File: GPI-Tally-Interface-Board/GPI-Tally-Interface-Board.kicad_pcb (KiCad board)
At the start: 2 copper layers, 155 x 90 mm, 44 parts, among them J1 DB25_Female, J2 DB25_Female, J20 AMP171826-4, J8 THD-20-R, SW1 SW_Push_45deg, SW10 SW_Push_45deg, SW11 SW_Push_45deg, SW12 SW_Push_45deg, SW13 SW_Push_45deg, SW14 SW_Push_45deg, SW15 SW_Push_45deg, SW16 SW_Push_45deg, SW2 SW_Push_45deg, SW3 SW_Push_45deg, SW4 SW_Push_45deg, SW5 SW_Push_45deg, SW6 SW_Push_45deg, SW7 SW_Push_45deg, SW8 SW_Push_45deg, SW9 SW_Push_45deg, U1 BOB-12009, U2 BOB-12009, U3 BOB-12009, U4 BOB-12009

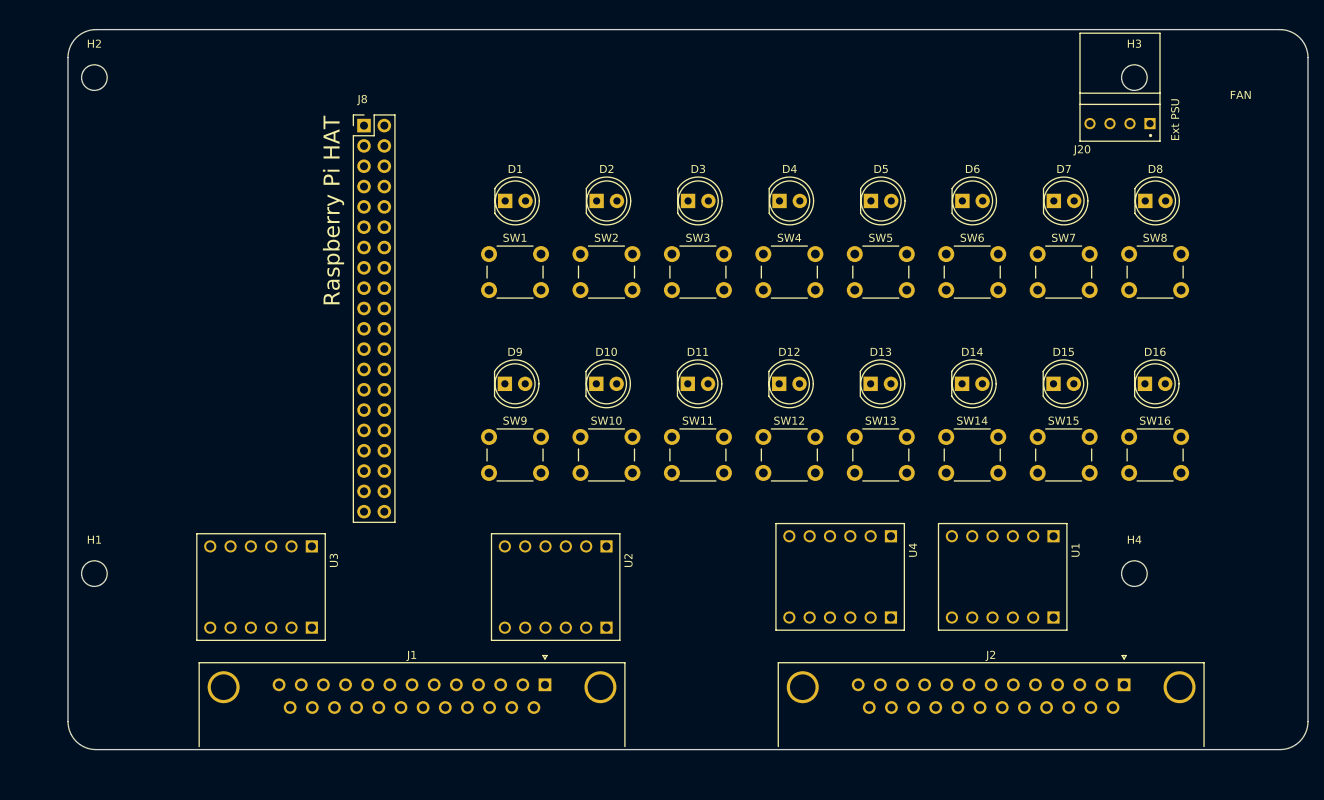
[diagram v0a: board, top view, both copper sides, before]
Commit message: oppto added
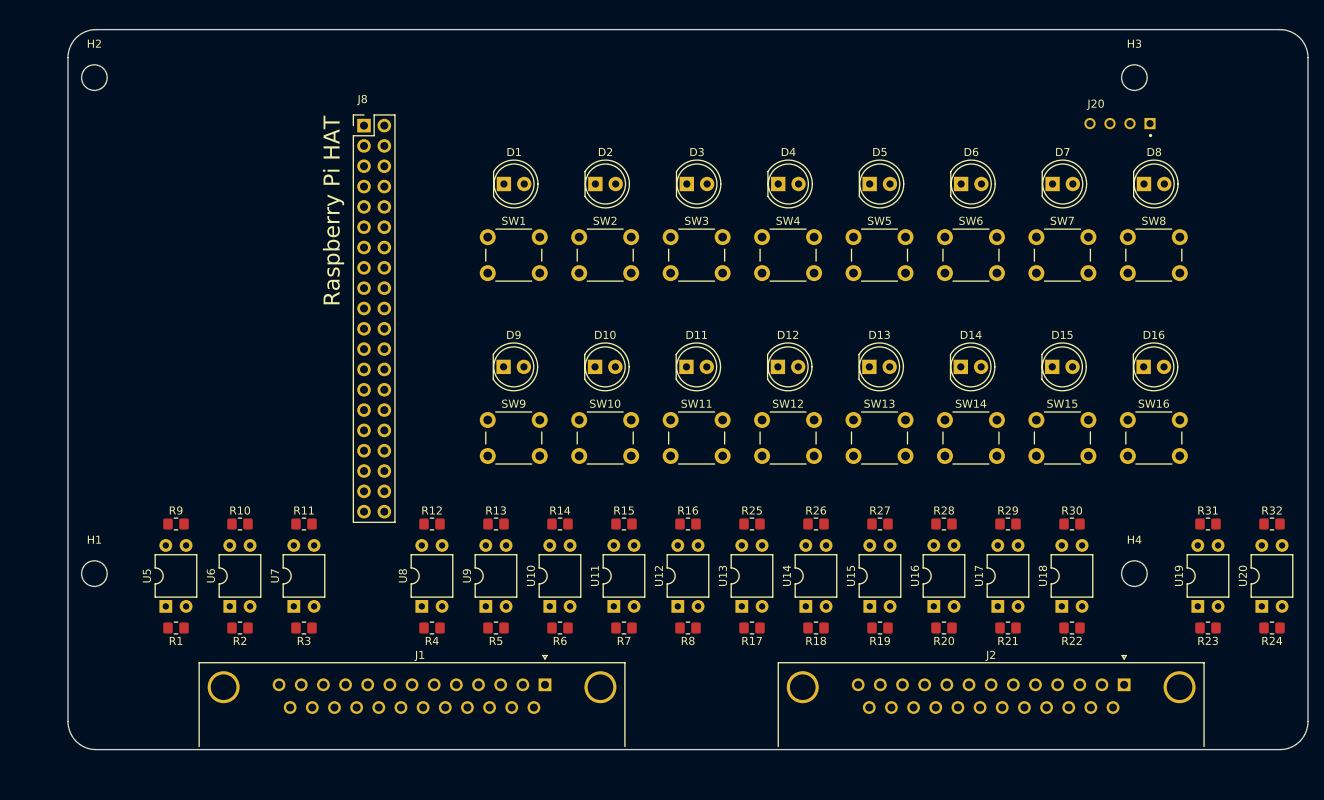
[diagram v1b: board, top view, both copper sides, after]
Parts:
- removed U1, U2, U3, U4: BOB-12009, BOB-12009:CONV_BOB-12009
- added R1: 470, Resistor_SMD:R_0805_2012Metric_Pad1.20x1.40mm_HandSolder, F.Cu at (77.0, 124.5)
- added R10: 470, Resistor_SMD:R_0805_2012Metric_Pad1.20x1.40mm_HandSolder, F.Cu at (85.0, 111.5)
- added R11: 470, Resistor_SMD:R_0805_2012Metric_Pad1.20x1.40mm_HandSolder, F.Cu at (93.0, 111.5)
- added R12: 470, Resistor_SMD:R_0805_2012Metric_Pad1.20x1.40mm_HandSolder, F.Cu at (109.0, 111.5)
- added R13: 470, Resistor_SMD:R_0805_2012Metric_Pad1.20x1.40mm_HandSolder, F.Cu at (117.0, 111.5)
- added R14: 470, Resistor_SMD:R_0805_2012Metric_Pad1.20x1.40mm_HandSolder, F.Cu at (125.0, 111.5)
- added R15: 470, Resistor_SMD:R_0805_2012Metric_Pad1.20x1.40mm_HandSolder, F.Cu at (133.0, 111.5)
- added R16: 470, Resistor_SMD:R_0805_2012Metric_Pad1.20x1.40mm_HandSolder, F.Cu at (141.0, 111.5)
- added R17: 470, Resistor_SMD:R_0805_2012Metric_Pad1.20x1.40mm_HandSolder, F.Cu at (149.0, 124.5)
- added R18: 470, Resistor_SMD:R_0805_2012Metric_Pad1.20x1.40mm_HandSolder, F.Cu at (157.0, 124.5)
- added R19: 470, Resistor_SMD:R_0805_2012Metric_Pad1.20x1.40mm_HandSolder, F.Cu at (165.0, 124.5)
- added R2: 470, Resistor_SMD:R_0805_2012Metric_Pad1.20x1.40mm_HandSolder, F.Cu at (85.0, 124.5)
- added R20: 470, Resistor_SMD:R_0805_2012Metric_Pad1.20x1.40mm_HandSolder, F.Cu at (173.0, 124.5)
- added R21: 470, Resistor_SMD:R_0805_2012Metric_Pad1.20x1.40mm_HandSolder, F.Cu at (181.0, 124.5)
- added R22: 470, Resistor_SMD:R_0805_2012Metric_Pad1.20x1.40mm_HandSolder, F.Cu at (189.0, 124.5)
- added R23: 470, Resistor_SMD:R_0805_2012Metric_Pad1.20x1.40mm_HandSolder, F.Cu at (206.0, 124.5)
- added R24: 470, Resistor_SMD:R_0805_2012Metric_Pad1.20x1.40mm_HandSolder, F.Cu at (214.0, 124.5)
- added R25: 470, Resistor_SMD:R_0805_2012Metric_Pad1.20x1.40mm_HandSolder, F.Cu at (149.0, 111.5)
- added R26: 470, Resistor_SMD:R_0805_2012Metric_Pad1.20x1.40mm_HandSolder, F.Cu at (157.0, 111.5)
- added R27: 470, Resistor_SMD:R_0805_2012Metric_Pad1.20x1.40mm_HandSolder, F.Cu at (165.0, 111.5)
- added R28: 470, Resistor_SMD:R_0805_2012Metric_Pad1.20x1.40mm_HandSolder, F.Cu at (173.0, 111.5)
- added R29: 470, Resistor_SMD:R_0805_2012Metric_Pad1.20x1.40mm_HandSolder, F.Cu at (181.0, 111.5)
- added R3: 470, Resistor_SMD:R_0805_2012Metric_Pad1.20x1.40mm_HandSolder, F.Cu at (93.0, 124.5)
- added R30: 470, Resistor_SMD:R_0805_2012Metric_Pad1.20x1.40mm_HandSolder, F.Cu at (189.0, 111.5)
- added R31: 470, Resistor_SMD:R_0805_2012Metric_Pad1.20x1.40mm_HandSolder, F.Cu at (206.0, 111.5)
- added R32: 470, Resistor_SMD:R_0805_2012Metric_Pad1.20x1.40mm_HandSolder, F.Cu at (214.0, 111.5)
- added R4: 470, Resistor_SMD:R_0805_2012Metric_Pad1.20x1.40mm_HandSolder, F.Cu at (109.0, 124.5)
- added R5: 470, Resistor_SMD:R_0805_2012Metric_Pad1.20x1.40mm_HandSolder, F.Cu at (117.0, 124.5)
- added R6: 470, Resistor_SMD:R_0805_2012Metric_Pad1.20x1.40mm_HandSolder, F.Cu at (125.0, 124.5)
- added R7: 470, Resistor_SMD:R_0805_2012Metric_Pad1.20x1.40mm_HandSolder, F.Cu at (133.0, 124.5)
- added R8: 470, Resistor_SMD:R_0805_2012Metric_Pad1.20x1.40mm_HandSolder, F.Cu at (141.0, 124.5)
- added R9: 470, Resistor_SMD:R_0805_2012Metric_Pad1.20x1.40mm_HandSolder, F.Cu at (77.0, 111.5)
- added U10: EL817, Package_DIP:DIP-4_W7.62mm, F.Cu at (123.7, 121.8)
- added U11: EL817, Package_DIP:DIP-4_W7.62mm, F.Cu at (131.7, 121.8)
- added U12: EL817, Package_DIP:DIP-4_W7.62mm, F.Cu at (139.7, 121.8)
- added U13: EL817, Package_DIP:DIP-4_W7.62mm, F.Cu at (147.7, 121.8)
- added U14: EL817, Package_DIP:DIP-4_W7.62mm, F.Cu at (155.7, 121.8)
- added U15: EL817, Package_DIP:DIP-4_W7.62mm, F.Cu at (163.7, 121.8)
- added U16: EL817, Package_DIP:DIP-4_W7.62mm, F.Cu at (171.7, 121.8)
- added U17: EL817, Package_DIP:DIP-4_W7.62mm, F.Cu at (179.7, 121.8)
- added U18: EL817, Package_DIP:DIP-4_W7.62mm, F.Cu at (187.7, 121.8)
- added U19: EL817, Package_DIP:DIP-4_W7.62mm, F.Cu at (204.7, 121.8)
- added U20: EL817, Package_DIP:DIP-4_W7.62mm, F.Cu at (212.7, 121.8)
- added U5: EL817, Package_DIP:DIP-4_W7.62mm, F.Cu at (75.7, 121.8)
- added U6: EL817, Package_DIP:DIP-4_W7.62mm, F.Cu at (83.7, 121.8)
- added U7: EL817, Package_DIP:DIP-4_W7.62mm, F.Cu at (91.7, 121.8)
- added U8: EL817, Package_DIP:DIP-4_W7.62mm, F.Cu at (107.7, 121.8)
- added U9: EL817, Package_DIP:DIP-4_W7.62mm, F.Cu at (115.7, 121.8)
- moved D13 2.13 mm to (163.7, 91.9)
- moved D2 2.13 mm to (129.4, 69.0)
- moved D6 2.13 mm to (175.1, 69.0)
- moved D1 2.13 mm to (118.0, 69.0)
- moved D10 2.13 mm to (129.4, 91.9)
- moved D11 2.13 mm to (140.8, 91.9)
- moved D12 2.13 mm to (152.2, 91.9)
- moved D14 2.13 mm to (175.1, 91.9)
- moved D15 2.13 mm to (186.5, 91.9)
- moved D16 2.13 mm to (198.0, 91.9)
- moved D3 2.13 mm to (140.8, 69.0)
- moved D4 2.13 mm to (152.3, 69.0)
- moved D5 2.13 mm to (163.7, 69.0)
- moved D7 2.13 mm to (186.6, 69.0)
- moved D8 2.13 mm to (198.0, 69.0)
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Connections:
- net +12v renamed /+12v
- J1 pad 1: GND -> GND1
- J1 pad 11: GND -> GND1
- J1 pad 12: GND -> GND1
- J1 pad 13: GND -> GND1
- J1 pad 14: GND -> GND1
- J1 pad 15: GND -> GND1
- J1 pad 2: GND -> GND1
- J1 pad 24: GND -> GND1
- J1 pad 25: GND -> GND1
- J2 pad 1: GND -> GND2
- J2 pad 11: GND -> GND2
- J2 pad 12: GND -> GND2
- J2 pad 13: GND -> GND2
- J2 pad 14: GND -> GND2
- J2 pad 15: GND -> GND2
- J2 pad 2: GND -> GND2
- J2 pad 24: GND -> GND2
- J2 pad 25: GND -> GND2
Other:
- board text removed: "Ext PSU"
- board text removed: "FAN"

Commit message: mirror
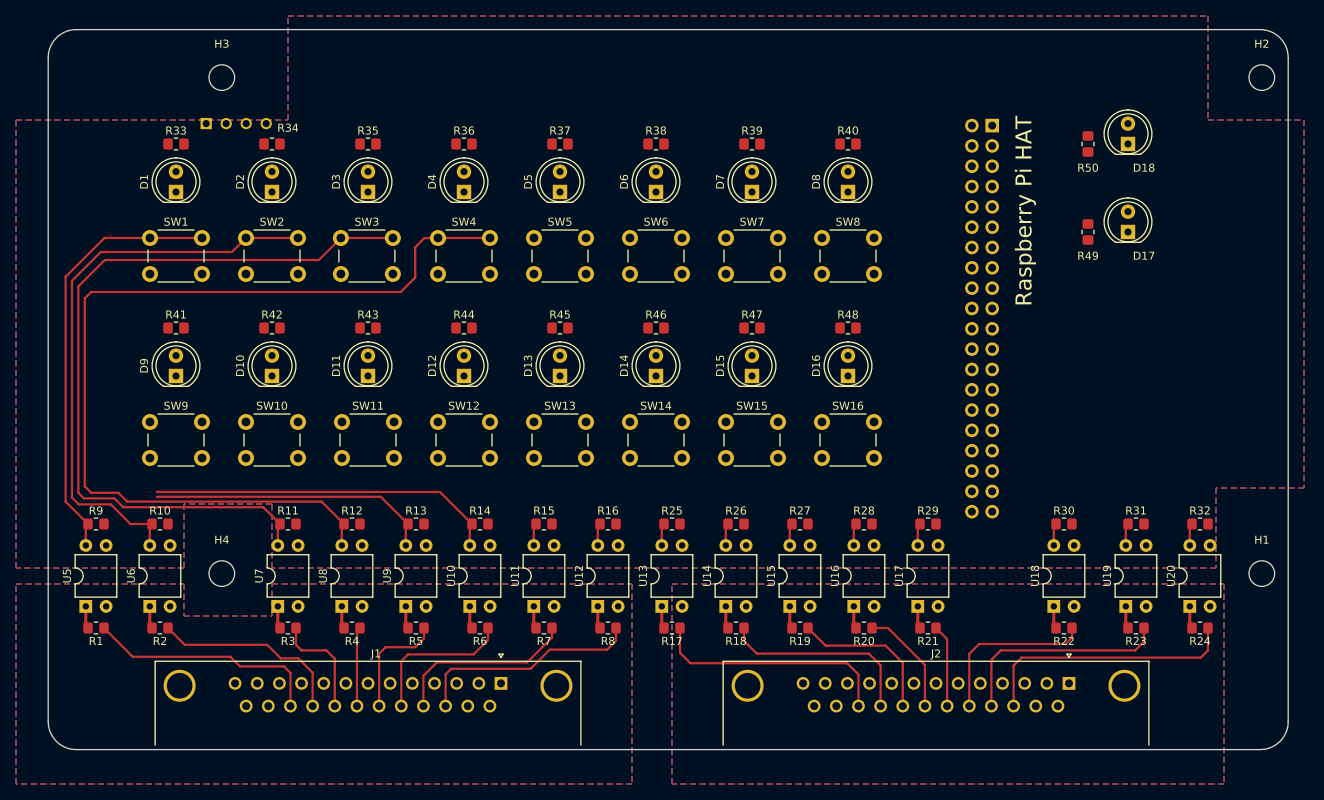
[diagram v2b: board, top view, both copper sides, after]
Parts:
- added D17: LED, LED_THT:LED_D5.0mm_IRGrey, F.Cu at (196.0, 75.0)
- added D18: LED, LED_THT:LED_D5.0mm_Clear, F.Cu at (196.0, 64.0)
- added R33: 330, Resistor_SMD:R_0805_2012Metric_Pad1.20x1.40mm_HandSolder, F.Cu at (77.0, 64.0)
- added R34: 330, Resistor_SMD:R_0805_2012Metric_Pad1.20x1.40mm_HandSolder, F.Cu at (89.0, 64.0)
- added R35: 330, Resistor_SMD:R_0805_2012Metric_Pad1.20x1.40mm_HandSolder, F.Cu at (101.0, 64.0)
- added R36: 330, Resistor_SMD:R_0805_2012Metric_Pad1.20x1.40mm_HandSolder, F.Cu at (113.0, 64.0)
- added R37: 330, Resistor_SMD:R_0805_2012Metric_Pad1.20x1.40mm_HandSolder, F.Cu at (125.0, 64.0)
- added R38: 330, Resistor_SMD:R_0805_2012Metric_Pad1.20x1.40mm_HandSolder, F.Cu at (137.0, 64.0)
- added R39: 330, Resistor_SMD:R_0805_2012Metric_Pad1.20x1.40mm_HandSolder, F.Cu at (149.0, 64.0)
- added R40: 330, Resistor_SMD:R_0805_2012Metric_Pad1.20x1.40mm_HandSolder, F.Cu at (161.0, 64.0)
- added R41: 330, Resistor_SMD:R_0805_2012Metric_Pad1.20x1.40mm_HandSolder, F.Cu at (77.0, 87.0)
- added R42: 330, Resistor_SMD:R_0805_2012Metric_Pad1.20x1.40mm_HandSolder, F.Cu at (89.0, 87.0)
- added R43: 330, Resistor_SMD:R_0805_2012Metric_Pad1.20x1.40mm_HandSolder, F.Cu at (101.0, 87.0)
- added R44: 330, Resistor_SMD:R_0805_2012Metric_Pad1.20x1.40mm_HandSolder, F.Cu at (113.0, 87.0)
- added R45: 330, Resistor_SMD:R_0805_2012Metric_Pad1.20x1.40mm_HandSolder, F.Cu at (125.0, 87.0)
- added R46: 330, Resistor_SMD:R_0805_2012Metric_Pad1.20x1.40mm_HandSolder, F.Cu at (137.0, 87.0)
- added R47: 330, Resistor_SMD:R_0805_2012Metric_Pad1.20x1.40mm_HandSolder, F.Cu at (149.0, 87.0)
- added R48: 330, Resistor_SMD:R_0805_2012Metric_Pad1.20x1.40mm_HandSolder, F.Cu at (161.0, 87.0)
- added R49: 330, Resistor_SMD:R_0805_2012Metric_Pad1.20x1.40mm_HandSolder, F.Cu at (191.0, 75.0)
- added R50: 330, Resistor_SMD:R_0805_2012Metric_Pad1.20x1.40mm_HandSolder, F.Cu at (191.0, 64.0)
- J20, J8: moved to B.Cu
- moved H1 145.9 mm to (212.7, 117.7)
- moved H2 145.9 mm to (212.7, 55.7)
- moved H3 114.1 mm to (82.7, 55.7)
- moved H4 114.1 mm to (82.7, 117.7)
- moved J20 110.5 mm to (84.5, 56.9), turned to 0 degrees
- moved J8 78.5 mm to (179.0, 61.7), turned to 180 degrees
- moved SW9 42.2 mm to (73.8, 98.8)
- moved SW1 42.2 mm to (73.8, 75.8)
- moved SW10 41.7 mm to (85.8, 98.8)
- moved SW2 41.7 mm to (85.8, 75.8)
- moved SW3 41.2 mm to (97.6, 75.8)
- moved SW11 41.1 mm to (97.8, 98.8)
- moved D1 41.0 mm to (77.0, 70.0), turned to 90 degrees
- moved D9 41.0 mm to (77.0, 93.0), turned to 90 degrees
- moved SW12 40.5 mm to (109.8, 98.8)
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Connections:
- D1 pad 1: unconnected-(D1-Pad1) -> GPIO2
- D1 pad 2: unconnected-(D1-Pad2) -> Net-(D1-Pad2)
- D10 pad 1: unconnected-(D10-Pad1) -> GPIO23
- D10 pad 2: unconnected-(D10-Pad2) -> Net-(D10-Pad2)
- D11 pad 1: unconnected-(D11-Pad1) -> GPIO24
- D11 pad 2: unconnected-(D11-Pad2) -> Net-(D11-Pad2)
- D12 pad 1: unconnected-(D12-Pad1) -> GPIO8
- D12 pad 2: unconnected-(D12-Pad2) -> Net-(D12-Pad2)
- D13 pad 1: unconnected-(D13-Pad1) -> GPIO11
- D13 pad 2: unconnected-(D13-Pad2) -> Net-(D13-Pad2)
- D14 pad 1: unconnected-(D14-Pad1) -> GPIO25
- D14 pad 2: unconnected-(D14-Pad2) -> Net-(D14-Pad2)
- D15 pad 1: unconnected-(D15-Pad1) -> GPIO9
- D15 pad 2: unconnected-(D15-Pad2) -> Net-(D15-Pad2)
- D16 pad 1: unconnected-(D16-Pad1) -> GPIO10
- D16 pad 2: unconnected-(D16-Pad2) -> Net-(D16-Pad2)
- D2 pad 1: unconnected-(D2-Pad1) -> GPIO3
- D2 pad 2: unconnected-(D2-Pad2) -> Net-(D2-Pad2)
- D3 pad 1: unconnected-(D3-Pad1) -> GPIO4
- D3 pad 2: unconnected-(D3-Pad2) -> Net-(D3-Pad2)
- D4 pad 1: unconnected-(D4-Pad1) -> GPIO14
- D4 pad 2: unconnected-(D4-Pad2) -> Net-(D4-Pad2)
- D5 pad 1: unconnected-(D5-Pad1) -> GPIO15
- D5 pad 2: unconnected-(D5-Pad2) -> Net-(D5-Pad2)
- D6 pad 1: unconnected-(D6-Pad1) -> GPIO18
- D6 pad 2: unconnected-(D6-Pad2) -> Net-(D6-Pad2)
- D7 pad 1: unconnected-(D7-Pad1) -> GPIO17
- D7 pad 2: unconnected-(D7-Pad2) -> Net-(D7-Pad2)
- D8 pad 1: unconnected-(D8-Pad1) -> GPIO27
- D8 pad 2: unconnected-(D8-Pad2) -> Net-(D8-Pad2)
- D9 pad 1: unconnected-(D9-Pad1) -> GPIO22
- D9 pad 2: unconnected-(D9-Pad2) -> Net-(D9-Pad2)
- R10 pad 1: Net-(U6-Pad4) -> GPIO3
- R11 pad 1: Net-(U7-Pad4) -> GPIO4
- R12 pad 1: Net-(U8-Pad4) -> GPIO14
- R13 pad 1: Net-(U9-Pad4) -> GPIO15
- R14 pad 1: Net-(U10-Pad4) -> GPIO18
- R15 pad 1: Net-(U11-Pad4) -> GPIO17
- R16 pad 1: Net-(U12-Pad4) -> GPIO27
- R25 pad 1: Net-(U13-Pad4) -> GPIO22
- R26 pad 1: Net-(U14-Pad4) -> GPIO23
- R27 pad 1: Net-(U15-Pad4) -> GPIO24
- R28 pad 1: Net-(U16-Pad4) -> GPIO10
- R29 pad 1: Net-(U17-Pad4) -> GPIO9
- R30 pad 1: Net-(U18-Pad4) -> GPIO25
- R31 pad 1: Net-(U19-Pad4) -> GPIO11
- R32 pad 1: Net-(U20-Pad4) -> GPIO8
- R9 pad 1: Net-(U5-Pad4) -> GPIO2
- SW1 pad 1: unconnected-(SW1-Pad1) -> GPIO2
- SW1 pad 2: unconnected-(SW1-Pad2) -> GND
- SW10 pad 1: unconnected-(SW10-Pad1) -> GPIO23
- SW10 pad 2: unconnected-(SW10-Pad2) -> GND
- SW11 pad 1: unconnected-(SW11-Pad1) -> GPIO24
- SW11 pad 2: unconnected-(SW11-Pad2) -> GND
- SW12 pad 1: unconnected-(SW12-Pad1) -> GPIO10
- SW12 pad 2: unconnected-(SW12-Pad2) -> GND
- SW13 pad 1: unconnected-(SW13-Pad1) -> GPIO9
- SW13 pad 2: unconnected-(SW13-Pad2) -> GND
- SW14 pad 1: unconnected-(SW14-Pad1) -> GPIO25
- SW14 pad 2: unconnected-(SW14-Pad2) -> GND
- SW15 pad 1: unconnected-(SW15-Pad1) -> GPIO11
- SW15 pad 2: unconnected-(SW15-Pad2) -> GND
- SW16 pad 1: unconnected-(SW16-Pad1) -> GPIO8
- SW16 pad 2: unconnected-(SW16-Pad2) -> GND
- SW2 pad 1: unconnected-(SW2-Pad1) -> GPIO3
- SW2 pad 2: unconnected-(SW2-Pad2) -> GND
- SW3 pad 1: unconnected-(SW3-Pad1) -> GPIO4
- SW3 pad 2: unconnected-(SW3-Pad2) -> GND
- SW4 pad 1: unconnected-(SW4-Pad1) -> GPIO14
- SW4 pad 2: unconnected-(SW4-Pad2) -> GND
- SW5 pad 1: unconnected-(SW5-Pad1) -> GPIO15
- SW5 pad 2: unconnected-(SW5-Pad2) -> GND
- SW6 pad 1: unconnected-(SW6-Pad1) -> GPIO18
- SW6 pad 2: unconnected-(SW6-Pad2) -> GND
- SW7 pad 1: unconnected-(SW7-Pad1) -> GPIO17
- SW7 pad 2: unconnected-(SW7-Pad2) -> GND
- SW8 pad 1: unconnected-(SW8-Pad1) -> GPIO27
- SW8 pad 2: unconnected-(SW8-Pad2) -> GND
- SW9 pad 1: unconnected-(SW9-Pad1) -> GPIO22
- SW9 pad 2: unconnected-(SW9-Pad2) -> GND
- U10 pad 4: Net-(U10-Pad4) -> GPIO18
- U11 pad 4: Net-(U11-Pad4) -> GPIO17
- U12 pad 4: Net-(U12-Pad4) -> GPIO27
- U13 pad 4: Net-(U13-Pad4) -> GPIO22
- U14 pad 4: Net-(U14-Pad4) -> GPIO23
- U15 pad 4: Net-(U15-Pad4) -> GPIO24
- U16 pad 4: Net-(U16-Pad4) -> GPIO10
- U17 pad 4: Net-(U17-Pad4) -> GPIO9
- U18 pad 4: Net-(U18-Pad4) -> GPIO25
- U19 pad 4: Net-(U19-Pad4) -> GPIO11
- U20 pad 4: Net-(U20-Pad4) -> GPIO8
- U5 pad 4: Net-(U5-Pad4) -> GPIO2
- U6 pad 4: Net-(U6-Pad4) -> GPIO3
- U7 pad 4: Net-(U7-Pad4) -> GPIO4
- U8 pad 4: Net-(U8-Pad4) -> GPIO14
- U9 pad 4: Net-(U9-Pad4) -> GPIO15
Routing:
- net GPIO14: track 0.00 -> 116.6 mm
- net GPIO4: track 0.00 -> 97.2 mm
- net GPIO3: track 0.00 -> 71.7 mm
- net GPIO2: track 0.00 -> 53.9 mm
- net GPIO18: track 0.00 -> 43.9 mm
- net GPIO15: track 0.00 -> 35.6 mm
- net B_GPI_OUT_8: track 0.00 -> 32.9 mm
- net B_GPI_OUT_1: track 0.00 -> 30.5 mm
- net A_GPI_OUT_1: track 0.00 -> 29.8 mm
- net A_GPI_OUT_8: track 0.00 -> 28.6 mm
- net B_GPI_OUT_7: track 0.00 -> 27.5 mm
- net B_GPI_OUT_2: track 0.00 -> 25.0 mm
- net A_GPI_OUT_2: track 0.00 -> 24.6 mm
- net A_GPI_OUT_7: track 0.00 -> 23.0 mm
- net B_GPI_OUT_6: track 0.00 -> 21.4 mm
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- added copper zone on B.Cu, net GND
- added copper zone on F.Cu, net GND
- added copper zone on B.Cu, net GND1
- added copper zone on F.Cu, net GND1
- added copper zone on B.Cu, net GND2
- added copper zone on F.Cu, net GND2
